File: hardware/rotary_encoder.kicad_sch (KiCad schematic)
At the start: 9 parts, among them U14 PEC11R-4215F-S0024

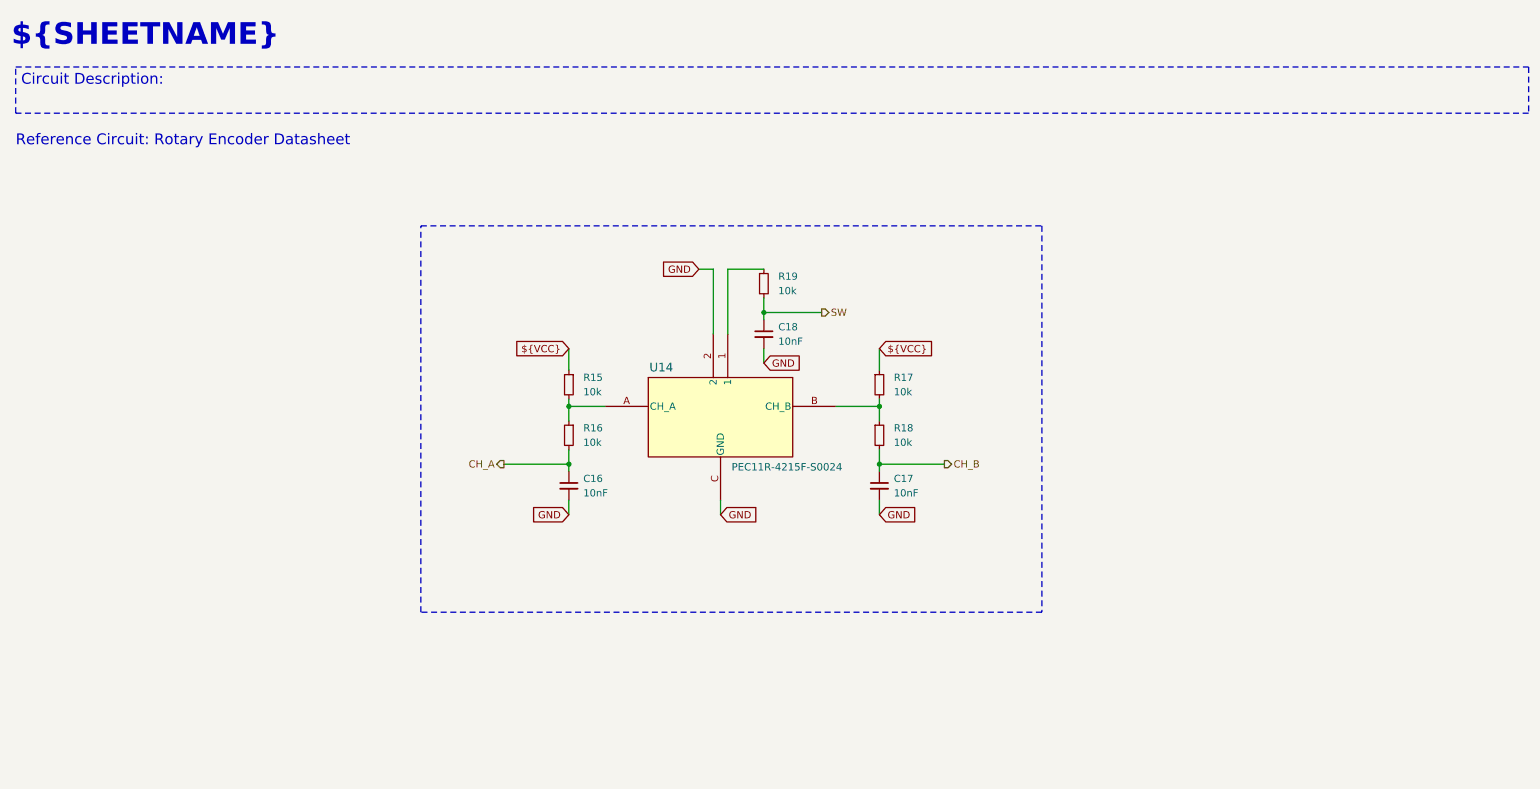
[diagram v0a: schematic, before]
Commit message: Electric Rules Check completed.
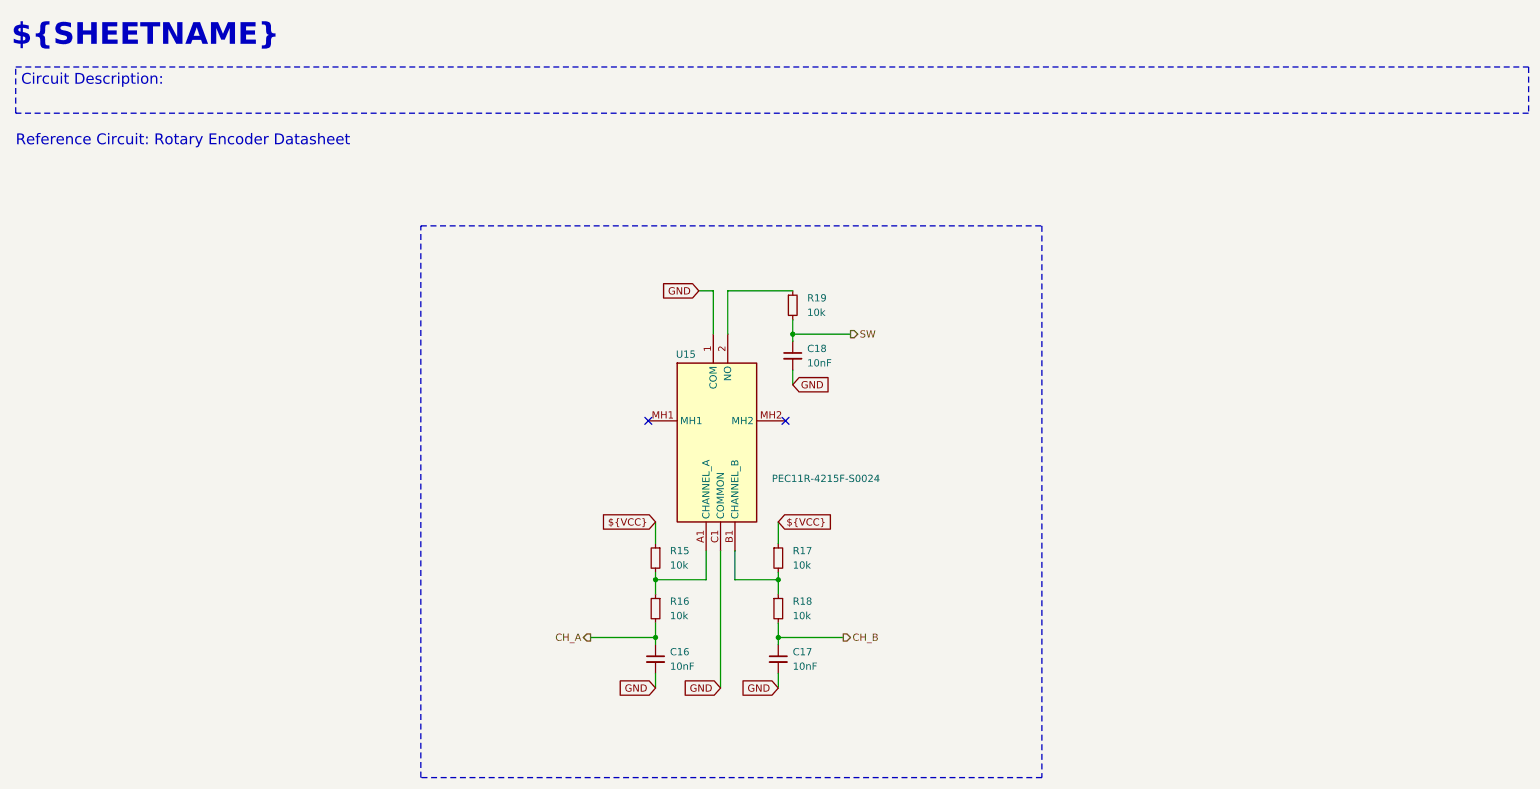
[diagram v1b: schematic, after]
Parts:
- removed U14: PEC11R-4215F-S0024, kitchen_timer:PEC11R4215FS0024, symbol kitchen_timer-symbols_lib:PEC11R-4215F-S0024
- added U15: PEC11R-4215F-S0024, kitchen_timer:PEC11R4215FS0024, symbol kitchen_timer-symbols_lib:PEC11R-4215F-S0024
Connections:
- net GND: now also U15.1 (COM), U15.C1 (COMMON)
- net at R17.2, R18.1: now also U15.B1 (CHANNEL_B)
- net at R19.1: now also U15.2 (NO)
- net at R15.2, R16.1: now also U15.A1 (CHANNEL_A)
- no-connect marks 0 -> 2
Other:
- moved on the sheet: C16, C17, C18, R15, R16, R17, R18, R19
